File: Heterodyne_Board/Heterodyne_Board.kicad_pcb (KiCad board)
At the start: 2 copper layers, 100 x 100 mm, 56 parts, among them J1 AVR-ISP-6, J2 Speaker, J3 SWITCH, J4 LED, J6 AudioJack2_Ground_Switch, SW1 SW_SPST, SW2 SW_SPST, U1 ATtiny85-20P, U2 TLV9054xD, U3 AP2112K-3.3, U4 LM386, U5 W25X40CLSN

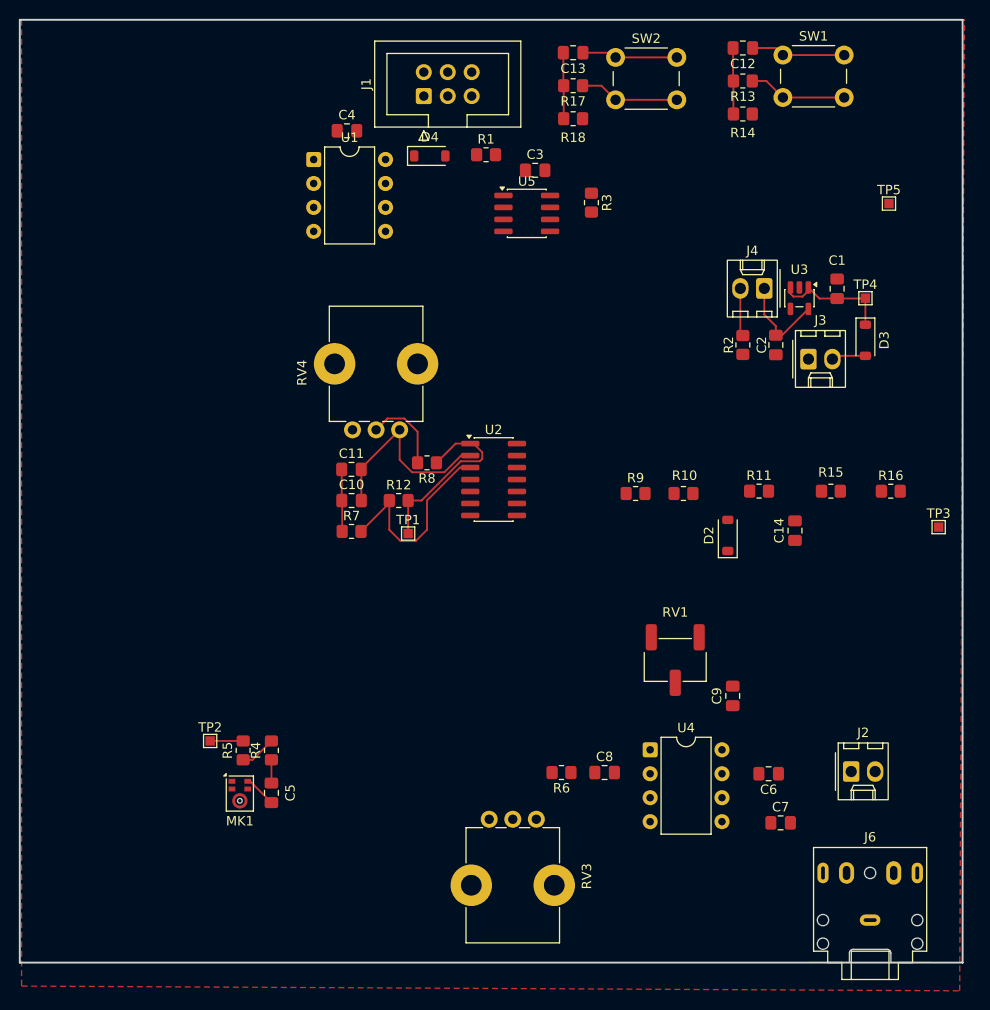
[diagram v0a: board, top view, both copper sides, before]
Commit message: Pushin P
done with routing!
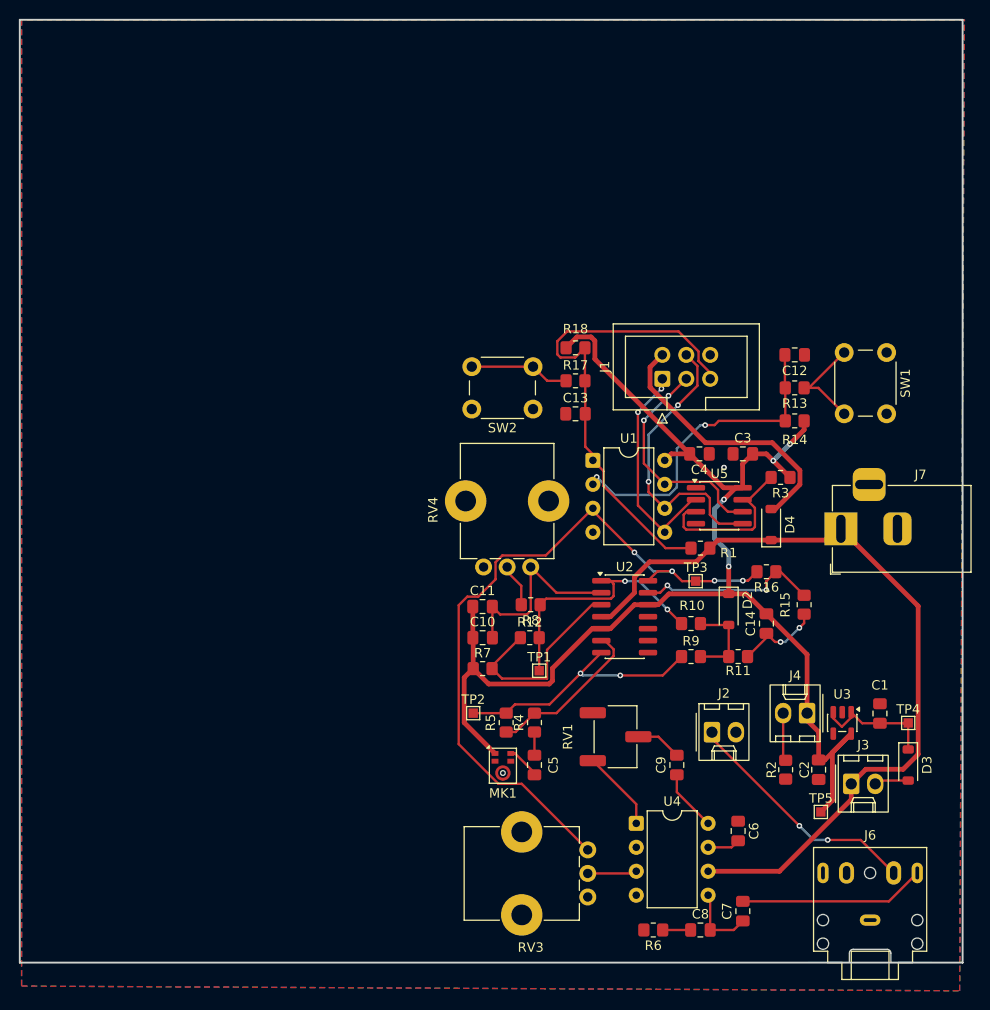
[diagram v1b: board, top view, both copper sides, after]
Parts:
- added J7: Barrel_Jack, Connector_BarrelJack:BarrelJack_Horizontal, F.Cu at (181.4, 84.0)
- moved TP5 64.9 mm to (179.3, 114.0)
- moved D4 53.3 mm to (174.0, 83.5), turned to 90 degrees
- moved C4 50.7 mm to (166.4, 76.0), turned to 180 degrees
- moved R1 47.5 mm to (166.5, 86.0), turned to 180 degrees
- moved C1 45.3 mm to (185.5, 103.6)
- moved TP4 45.3 mm to (188.5, 104.6)
- moved U3 45.3 mm to (181.5, 104.6)
- moved C2 45.3 mm to (179.0, 109.5)
- moved D3 45.3 mm to (188.5, 109.0)
- moved J3 45.3 mm to (182.5, 111.0)
- moved J4 45.3 mm to (177.8, 103.5)
- moved R2 45.3 mm to (175.5, 109.5)
- moved U1 43.5 mm to (155.1, 76.7)
- moved J1 39.2 mm to (162.5, 68.1)
- moved SW2 38.3 mm to (148.8, 71.3), turned to 180 degrees
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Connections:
- D4 pad 1: Net-(D4-K) -> +6V
- D4 pad 2: +5V -> Net-(D4-A)
- J1 pad 2: Net-(D4-K) -> Net-(D4-A)
- R1 pad 1: +5V -> +6V
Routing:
- net +3V3: track 16.7 -> 144.8 mm, vias 0 -> 4
- net +6V: track 0.00 -> 86.0 mm
- net /Speaker_in: track 0.00 -> 76.8 mm, vias 0 -> 4
- net /RESET: track 7.02 -> 52.1 mm
- net /MOSI: track 0.00 -> 30.9 mm, vias 0 -> 2
- net Net-(D4-A): track 0.00 -> 29.2 mm
- net /Audio_EN: track 7.02 -> 34.4 mm, vias 0 -> 2
- net Net-(J2-Pin_1): track 0.00 -> 25.8 mm, vias 0 -> 2
- net /SCK: track 0.00 -> 24.4 mm, vias 0 -> 2
- net /Mic_out: track 3.50 -> 27.9 mm, vias 0 -> 2
- net /MISO: track 0.00 -> 23.6 mm, vias 0 -> 2
- net Net-(C7-Pad2): track 0.00 -> 19.7 mm
- net Net-(U2D--): track 0.00 -> 19.5 mm, vias 0 -> 2
- net GND: track 20.2 -> 0.71 mm, vias 0 -> 1
- net Net-(U5-~{HOLD}): track 0.00 -> 18.2 mm
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- added copper zone on B.Cu, net GND
